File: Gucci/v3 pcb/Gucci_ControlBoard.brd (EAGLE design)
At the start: 66 x 56 mm, 78 parts, among them U1 PCA9306_LSSOP, U2 TEENSY_3.6_DIL, U5 LM393-8-SOIC, U6 AP2114H-1.8TRG1, U7 AP2114H-3.3TRG1

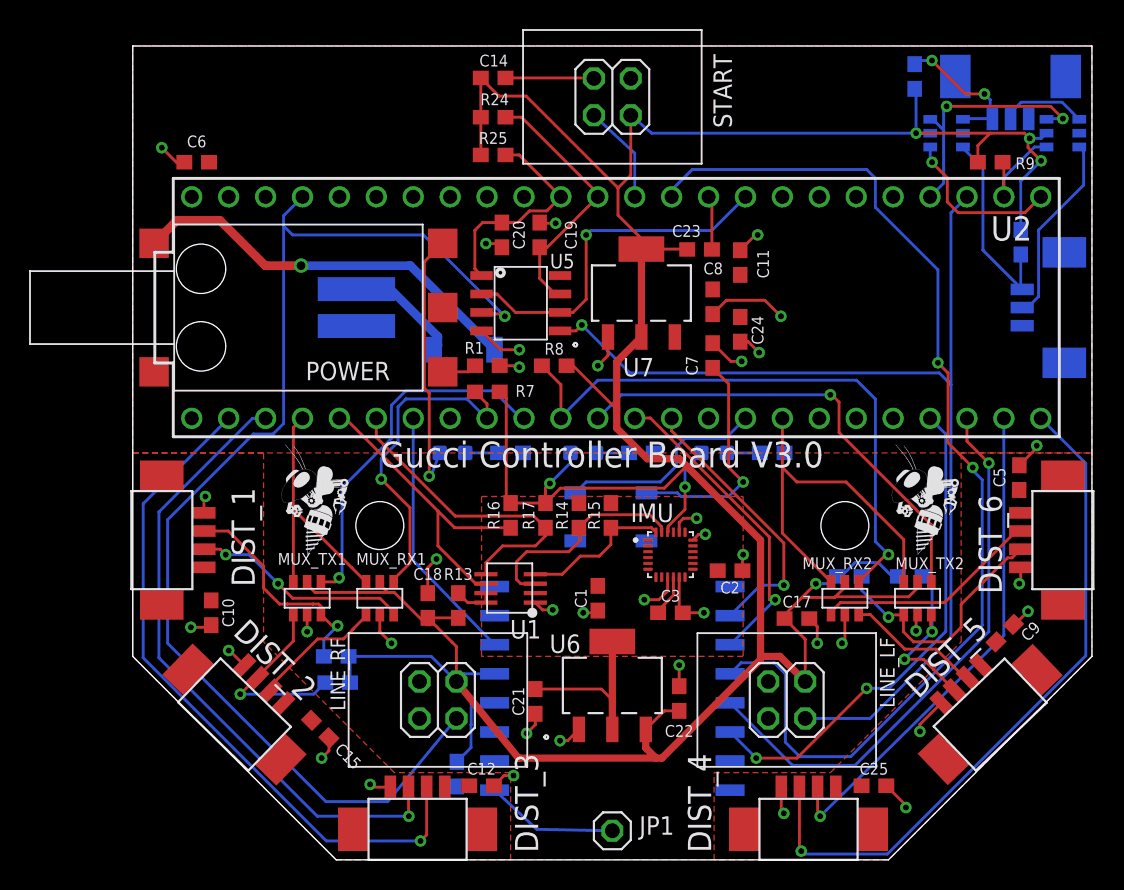
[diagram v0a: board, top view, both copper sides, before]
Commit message: Fixed Clearances  - Changed DRC
Fixed Clearance  - Changed DRC (JLCPCB Layer 2)
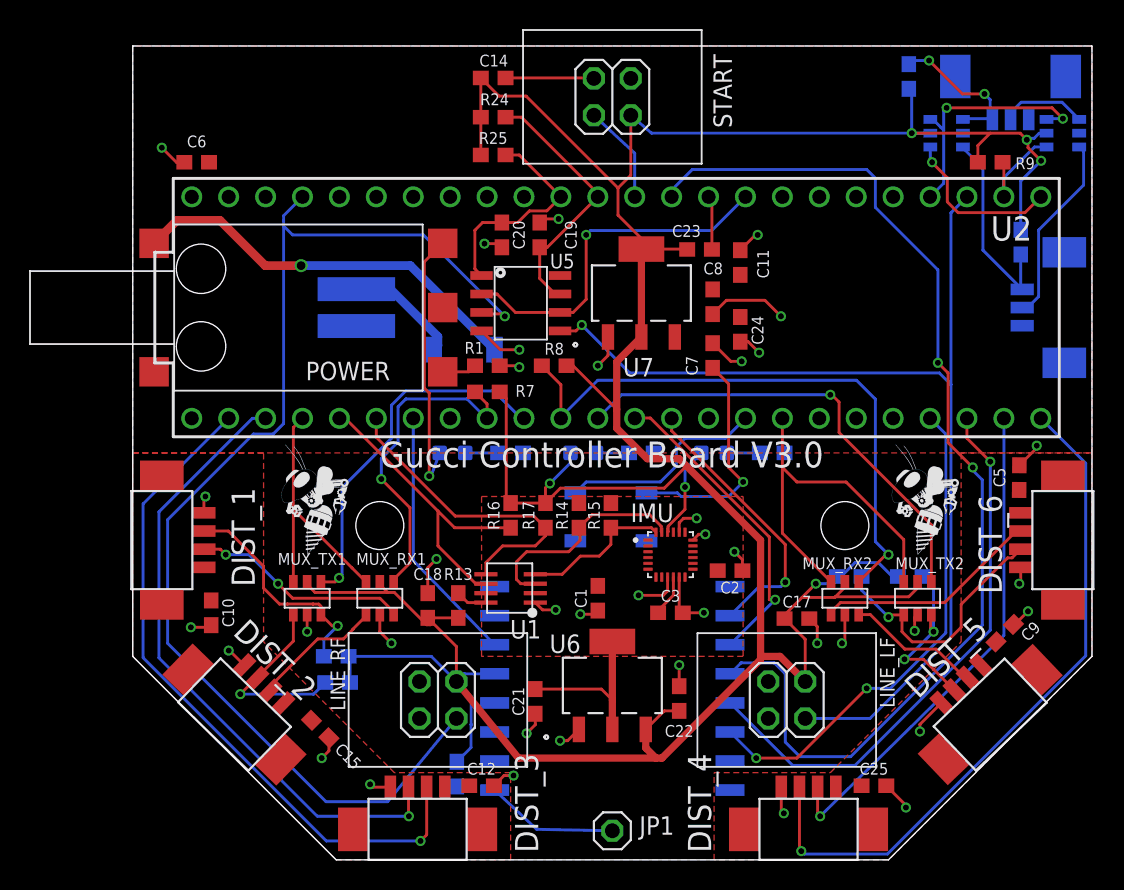
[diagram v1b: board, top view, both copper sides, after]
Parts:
- moved R11 0.40 mm to (39.4, 53.9)
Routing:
- net GND: track 81.2 -> 82.8 mm
